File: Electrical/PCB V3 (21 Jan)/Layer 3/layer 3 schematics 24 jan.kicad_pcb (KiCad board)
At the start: 2 copper layers, 181.6 x 151.3 mm, 22 parts, among them J1 Conn_01x06, J2 Conn_01x02, J3 Conn_01x06, J4 Conn_01x06, J5 Conn_01x06, J7 Conn_01x08, J8 Conn_01x02, U2 XT30UPB-M, U3 4754

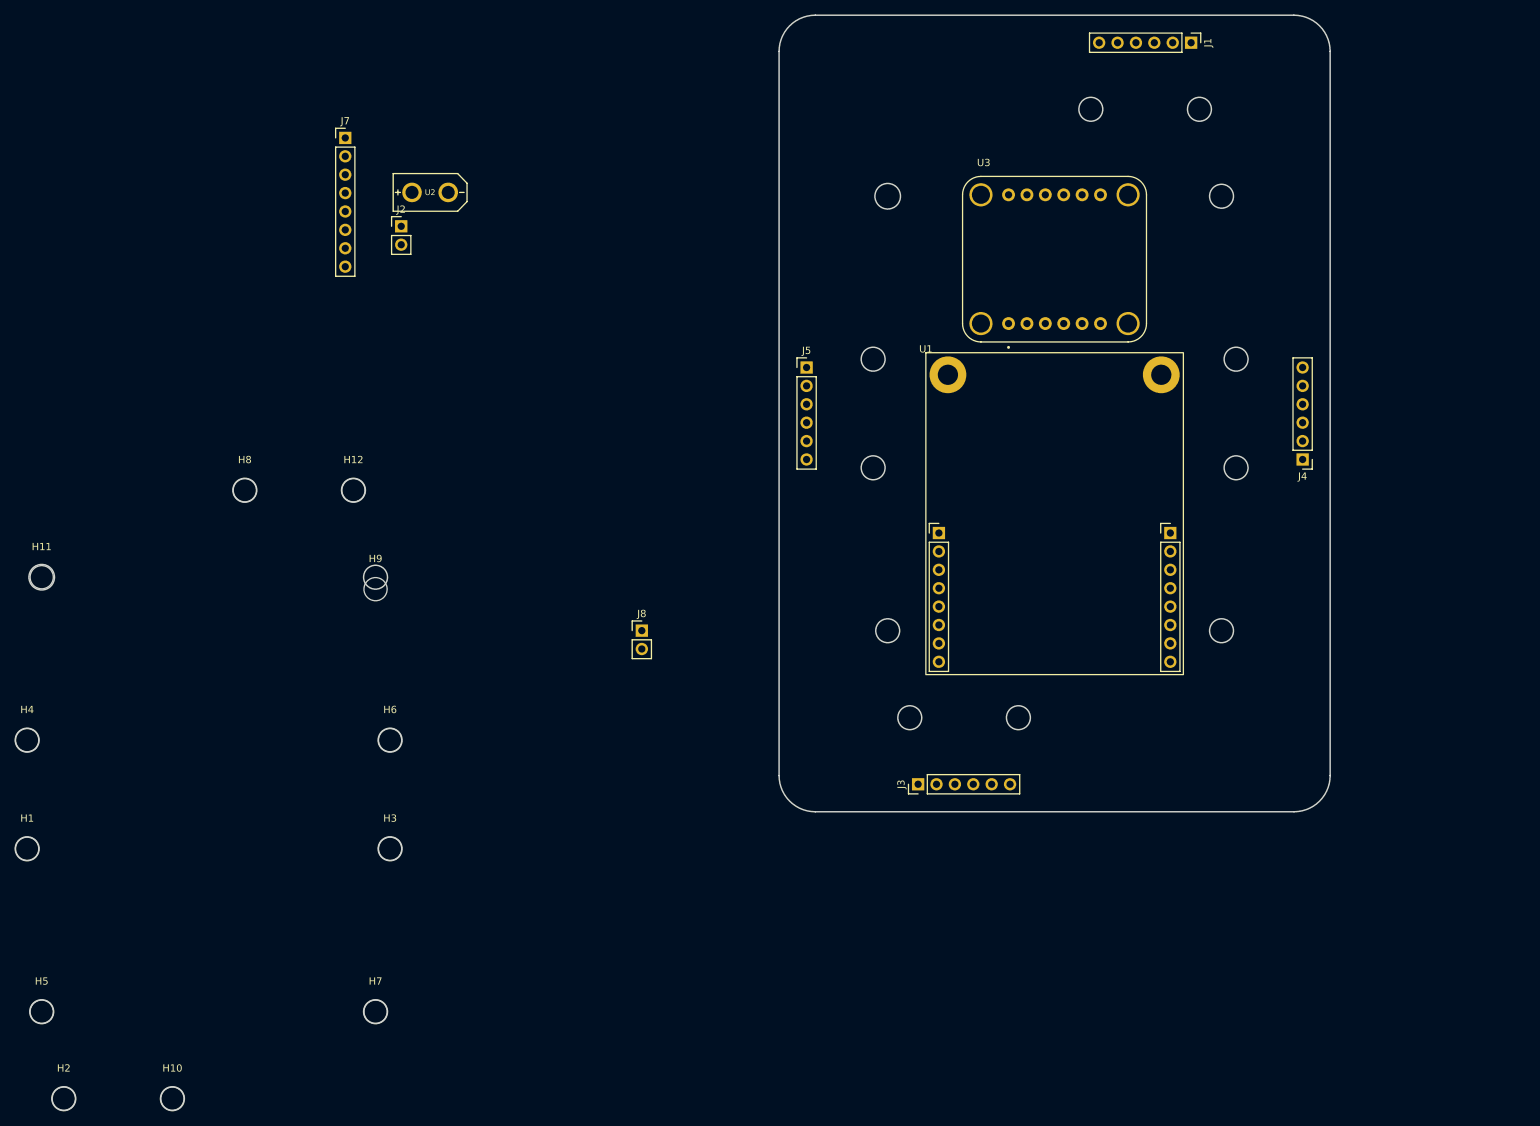
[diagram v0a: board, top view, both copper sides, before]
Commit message: 7 feb update!!! stop at pull up res
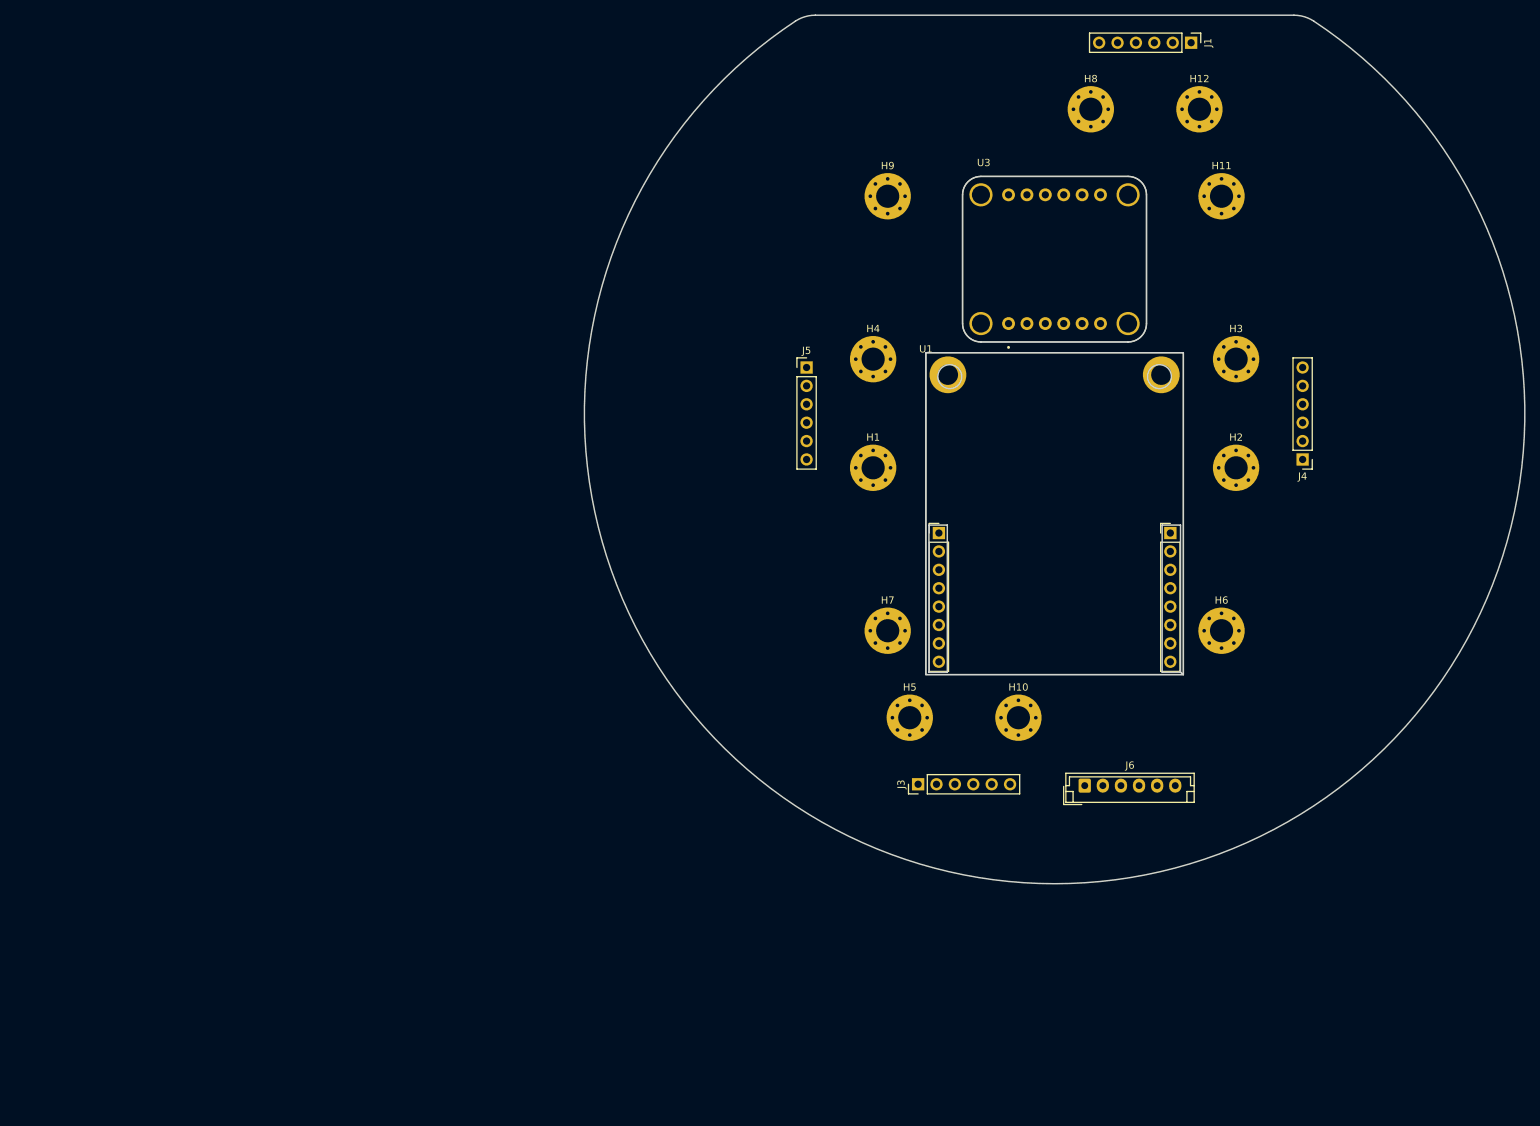
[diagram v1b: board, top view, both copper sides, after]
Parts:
- removed J2, J8: Conn_01x02, Connector_PinHeader_2.54mm:PinHeader_1x02_P2.54mm_Vertical
- removed J7: Conn_01x08, Connector_PinHeader_2.54mm:PinHeader_1x08_P2.54mm_Vertical
- removed U2: XT30UPB-M, XT30UPB-M:XT30UPB-M
- added J6: Conn_01x06, Connector_JST:JST_EH_B6B-EH-A_1x06_P2.50mm_Vertical, F.Cu at (217.9, 138.9)
- H1, H10, H11, H12, H2, H3, H4, H5, H6, H7, H8, H9: footprint MountingHole:MountingHole_3.2mm_M3 -> MountingHole:MountingHole_3.2mm_M3_Pad_Via
- moved H2 183.8 mm to (238.8, 95.0)
- moved H11 171.2 mm to (236.8, 57.5)
- moved H3 135.0 mm to (238.8, 80.0)
- moved H1 128.1 mm to (188.7, 95.0)
- moved H10 128.1 mm to (208.7, 129.5)
- moved H12 128.1 mm to (233.7, 45.5)
- moved H4 128.1 mm to (188.7, 80.0)
- moved H8 128.1 mm to (218.7, 45.5)
- moved H5 126.6 mm to (193.7, 129.5)
- moved H6 115.8 mm to (236.8, 117.5)
- moved H9 89.1 mm to (190.7, 57.5)
- moved H7 88.1 mm to (190.7, 117.5)
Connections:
- net /3V3 renamed +3V3
- net /GND renamed GND
- U1 pad 1: /RX -> /L3 RX
- U1 pad 2: /TX -> /L3 TX
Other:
- board size 181.6 x 151.3 mm -> 129.9 x 119.9 mm
